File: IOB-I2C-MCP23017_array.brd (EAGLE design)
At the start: 108.7 x 112 mm, 33 parts, among them IC1X11 MCP23017SO, IC1X12 MCP23017SO, IC1X13 MCP23017SO

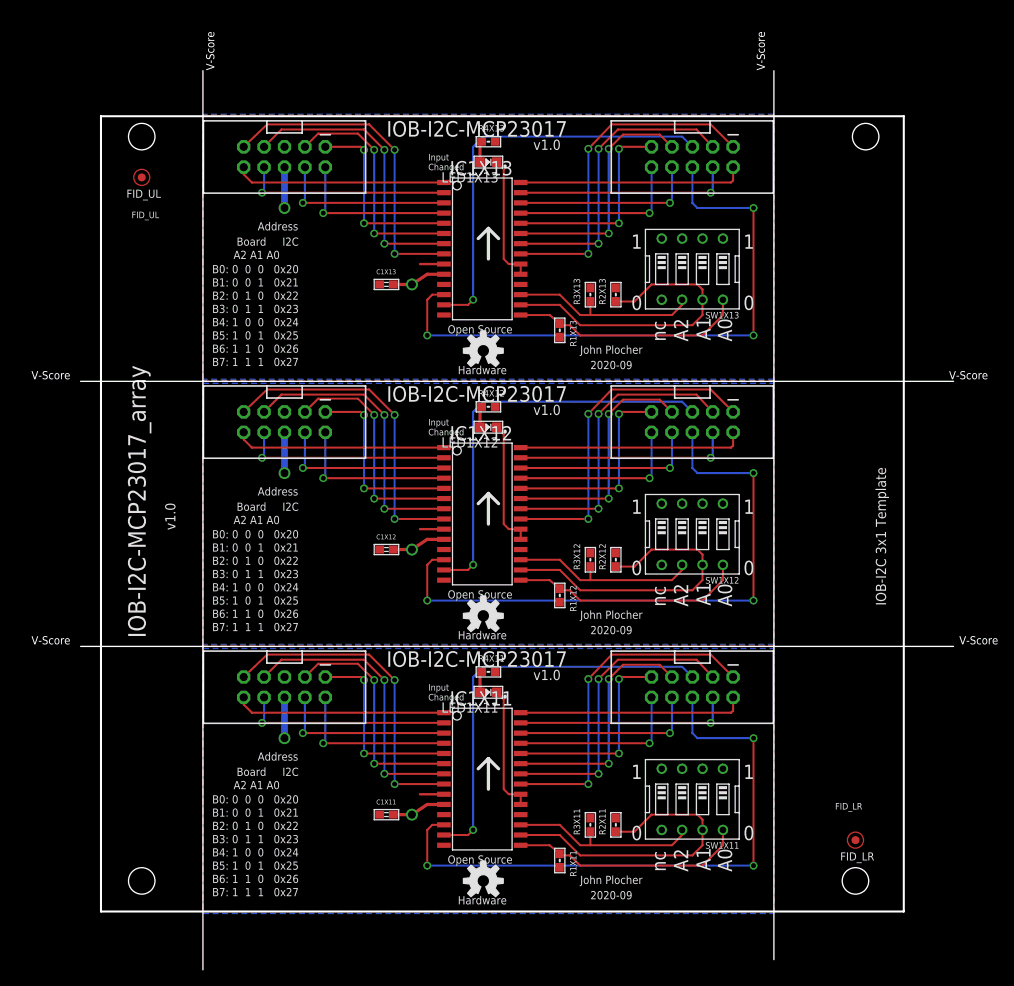
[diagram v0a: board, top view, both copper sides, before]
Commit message: cleanup layout
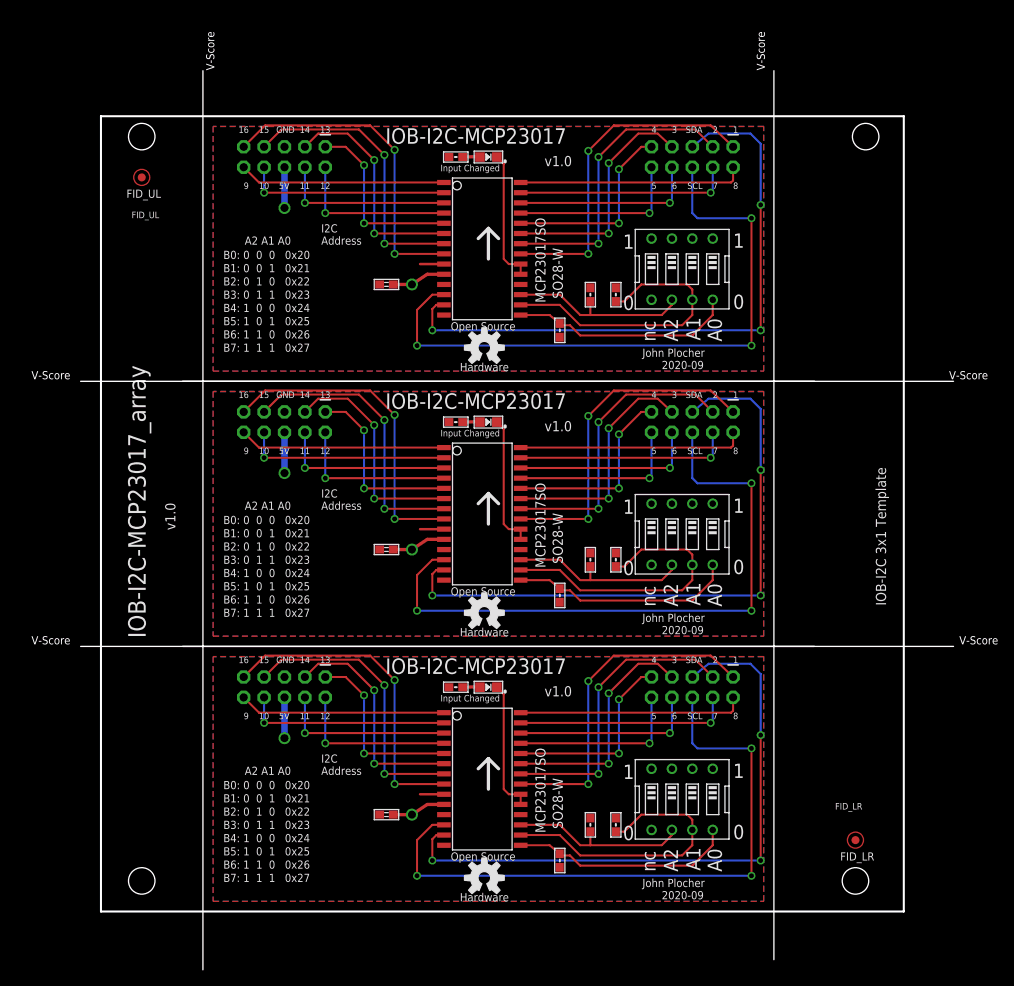
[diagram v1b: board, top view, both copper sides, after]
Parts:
- BOARDX11, BOARDX12, BOARDX13: value I2C-EXPANDER -> CONNECTOR-I2C-EXPANDER
- LED1X11, LED1X12, LED1X13: value (none) -> G
- R4X11, R4X12, R4X13: value 2k2 -> 4k7
- moved R4X12 4.49 mm to (44.2, 61.0), turned to 180 degrees
- moved R4X13 4.49 mm to (44.2, 94.0), turned to 180 degrees
- moved R4X11 4.49 mm to (44.2, 27.9), turned to 180 degrees
- moved SW1X11 1.27 mm to (72.4, 14.0)
- moved SW1X12 1.27 mm to (72.4, 47.0)
- moved SW1X13 1.27 mm to (72.4, 80.0)
- moved LED1X13 0.64 mm to (48.3, 94.0)
- moved LED1X11 0.64 mm to (48.3, 27.9)
- moved LED1X12 0.63 mm to (48.3, 61.0)
- moved OSHW1X12 0.40 mm to (47.8, 37.2)
- moved OSHW1X13 0.40 mm to (47.8, 70.2)
- moved OSHW1X11 0.40 mm to (47.8, 4.19)
- renumbered U$5X11 to BOARDX11, U$5X12 to BOARDX12, U$5X13 to BOARDX13
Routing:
- net SDAX12: track 51.3 -> 78.1 mm, vias 1 -> 3
- net SDAX11: track 51.3 -> 78.1 mm, vias 1 -> 3
- net SDAX13: track 51.3 -> 78.1 mm, vias 1 -> 3
- net SCLX12: track 75.6 -> 79.5 mm
- net SCLX13: track 75.6 -> 79.5 mm
- net SCLX11: track 75.6 -> 79.5 mm
- net A1X12: track 39.3 -> 36.8 mm
- net A1X11: track 39.3 -> 36.8 mm
- net A1X13: track 39.3 -> 36.8 mm
- net P4X13: track 25.7 -> 24.2 mm
- net P4X12: track 25.7 -> 24.2 mm
- net P4X11: track 25.7 -> 24.2 mm
- net A3X13: track 24.0 -> 22.7 mm
- net A0X12: track 29.1 -> 27.9 mm
- net A0X11: track 29.1 -> 27.9 mm
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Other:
- board text added: "BOARD"
- board text added: "I2C Address"
- board text added: "MCP23017SO"
- board text added: "SO28-W"
- board text removed: "Address"
- board text removed: "Board I2C"
- board text removed: "U$5"

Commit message: added values for connectors
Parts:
- FID_LR, FID_UL: value (none) -> FIDUCIAL
- U$5X1: value (none) -> 10x10
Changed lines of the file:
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@@
 <attribute name="VALUE" x="78.232" y="86.614" size="0.8128" layer="27" ratio="10" rot="R180"/>
 </element>
-<element name="U$5X1" library="SPCoast" package="BOARD-TEMPLATE-IOB-I2C-3X1-ARRAY" value="" x="0" y="0"/>
-<element name="FID_UL" library="SPCoast" package="FIDUCIAL_1MM" value="" x="5.08" y="91.44"/>
-<element name="FID_LR" library="SPCoast" package="FIDUCIAL_1MM" value="" x="93.98" y="8.89"/>
+<element name="U$5X1" library="SPCoast" package="BOARD-TEMPLATE-IOB-I2C-3X1-ARRAY" value="10x10" x="0" y="0"/>
+<element name="FID_UL" library="SPCoast" package="FIDUCIAL_1MM" value="FIDUCIAL" x="5.08" y="91.44"/>
+<element name="FID_LR" library="SPCoast" package="FIDUCIAL_1MM" value="FIDUCIAL" x="93.98" y="8.89"/>
 </elements>
 <signals>
